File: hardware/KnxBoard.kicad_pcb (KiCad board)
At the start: 4 copper layers, 40 parts, among them J1 Conn_01x10, J2 Conn_01x12, J3 Conn_01x12, J4 Conn_01x02_Male, SW1 SW_Push, SW2 SW_Push, U1 NCN5130, U2 STM32L432KCUx, X1 FA-238

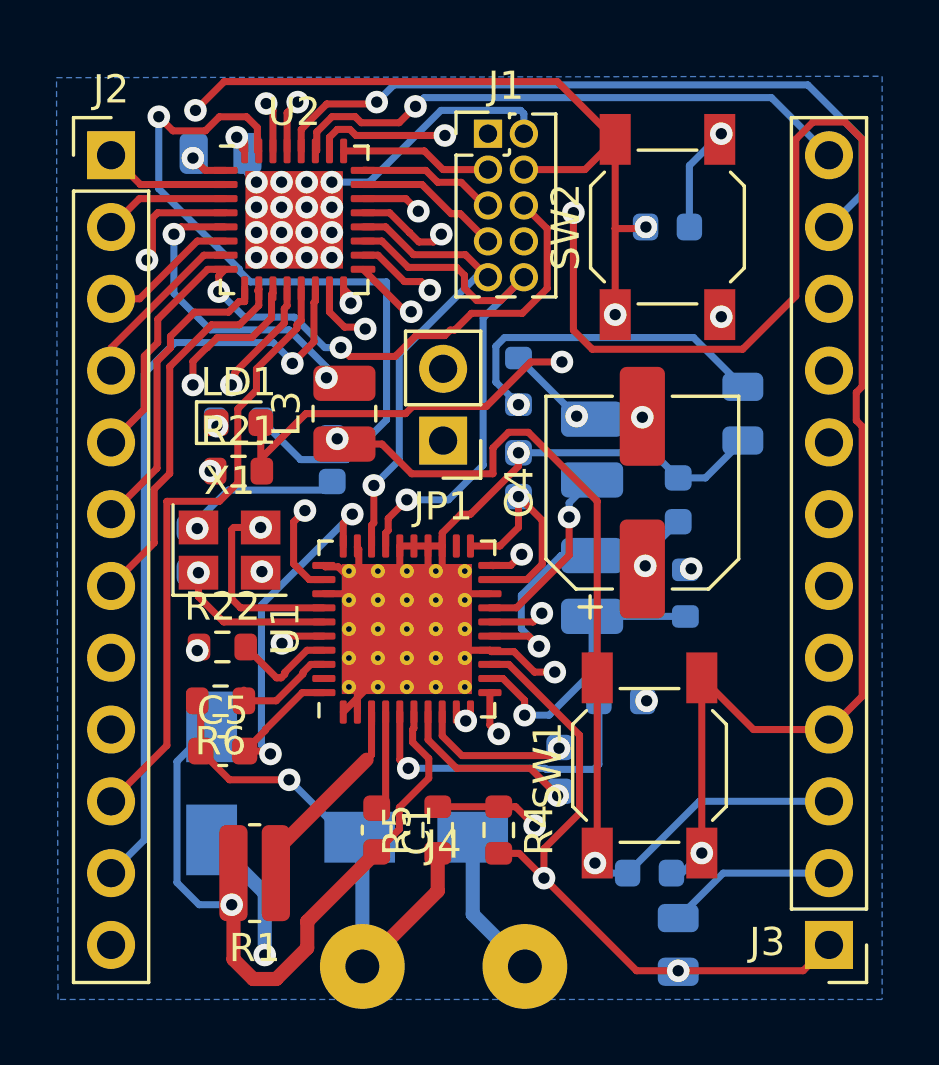
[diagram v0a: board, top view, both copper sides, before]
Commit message: Pad thermique
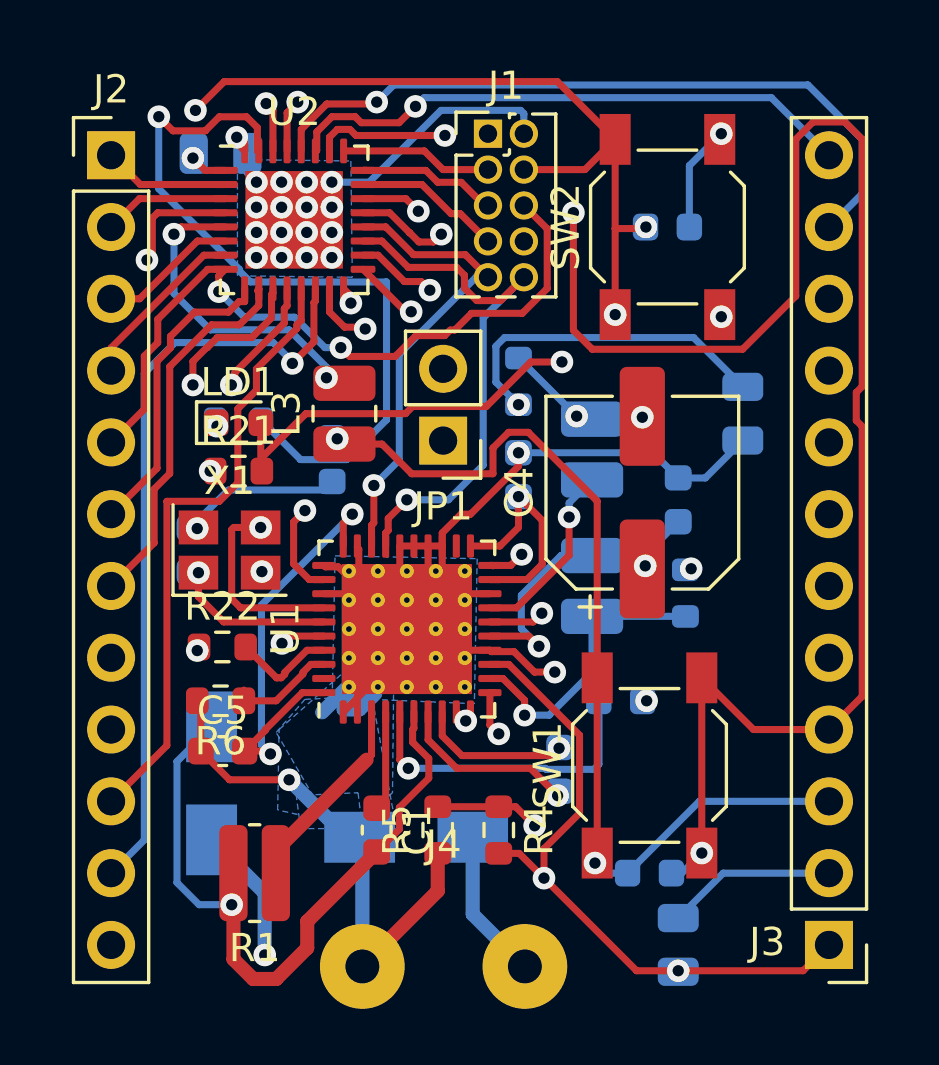
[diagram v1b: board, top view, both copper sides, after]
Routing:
- net GND: track 185.9 -> 200.2 mm
